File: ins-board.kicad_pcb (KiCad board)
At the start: 4 copper layers, 50 x 23 mm, 93 parts, among them P1 POWER, Q1 FDN306P, Q2 FDC638APZ, U1 24LC128, U10 HMC5883L, U11 H3LIS331DL, U2 STM32F415RGT6, U3 LTC4412, U4 MAX3051, U5 LT1965, U6 LT1761-3.3, U7 LT1965, U8 MS5611-01BA, U9 MPU6000, X1 CRYSTAL 16MHz 10ppm

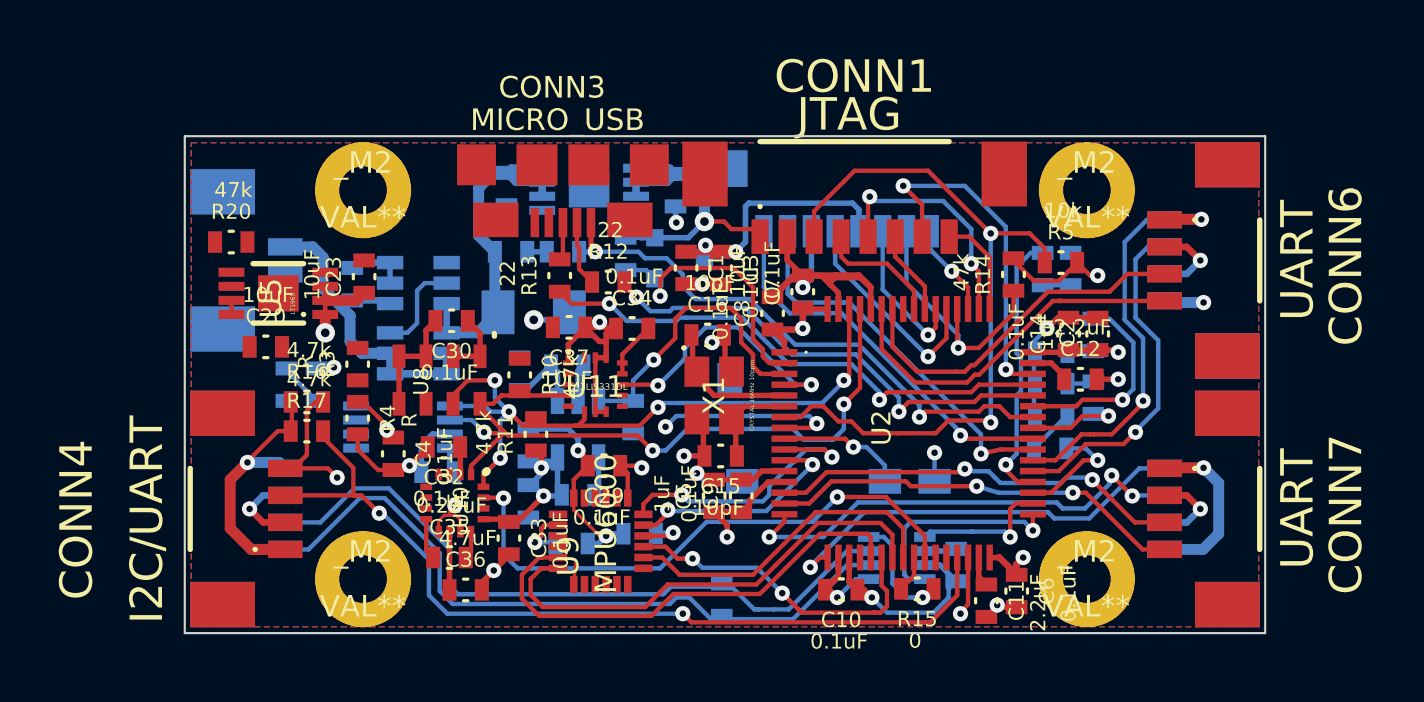
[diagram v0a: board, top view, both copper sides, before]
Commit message: routing (io_en)
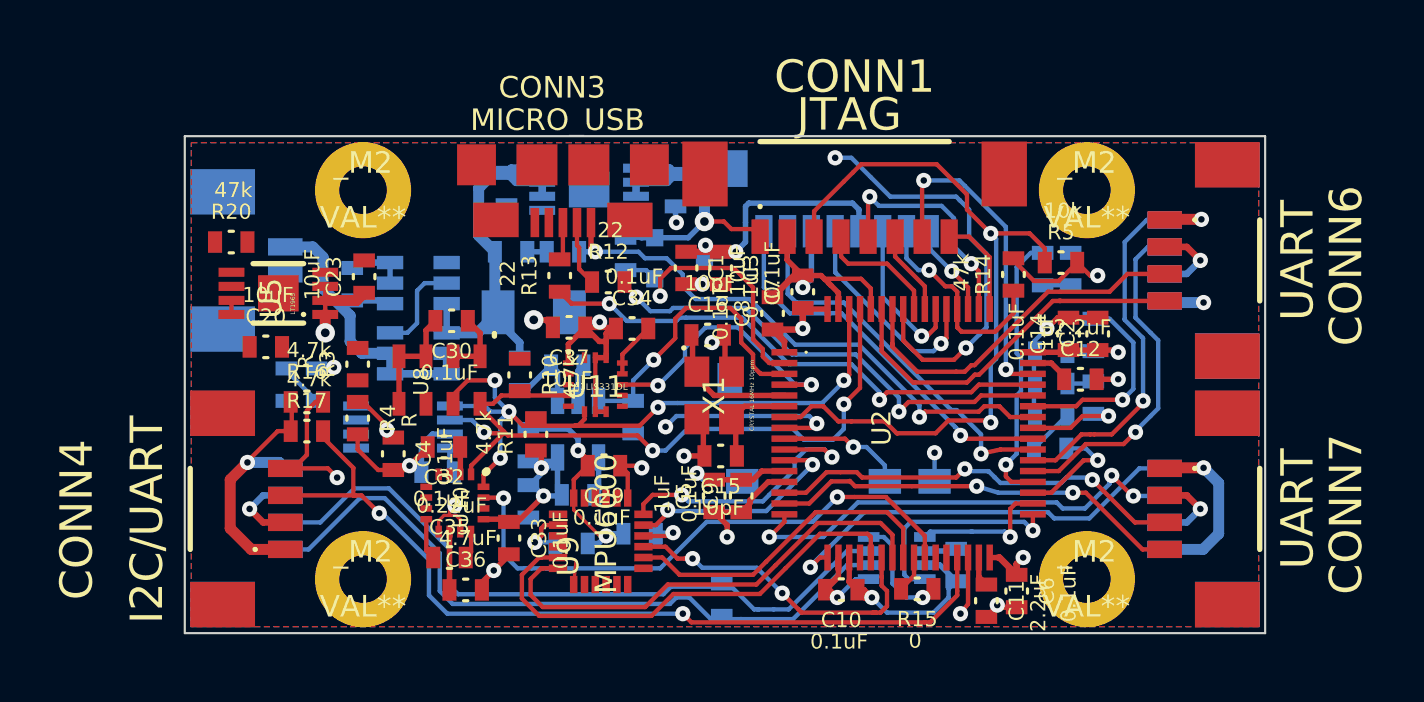
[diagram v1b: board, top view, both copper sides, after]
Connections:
- U2 pad 28: /IO_EN -> (no net)
- U2 pad 57: (no net) -> /IO_EN
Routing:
- net /IO_EN: track 0.00 -> 46.9 mm, vias 0 -> 2
- net GND: track 95.4 -> 92.6 mm
- net /V_IN: track 16.7 -> 19.2 mm
- net /SDIO_D3: track 12.5 -> 9.98 mm
- net /STM32F4_TMS: track 16.2 -> 15.3 mm
- net /STM32F4_NRST: track 34.2 -> 35.1 mm
